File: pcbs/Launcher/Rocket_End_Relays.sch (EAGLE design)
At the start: 39 parts, among them IC2 LM2576T-ADJ, K4 LD105, K5 LD105, K6 LD105, K7 LD105, T1 BC547, T2 BC547, T3 BC547, T4 BC547, T5 BC547, U1 ARDUINO-MEGAPRO-5V, X1 22-23-2041, X2 22-23-2041, X3 22-23-2021, X4 22-23-2021, X5 22-23-2021, X7 22-23-2021

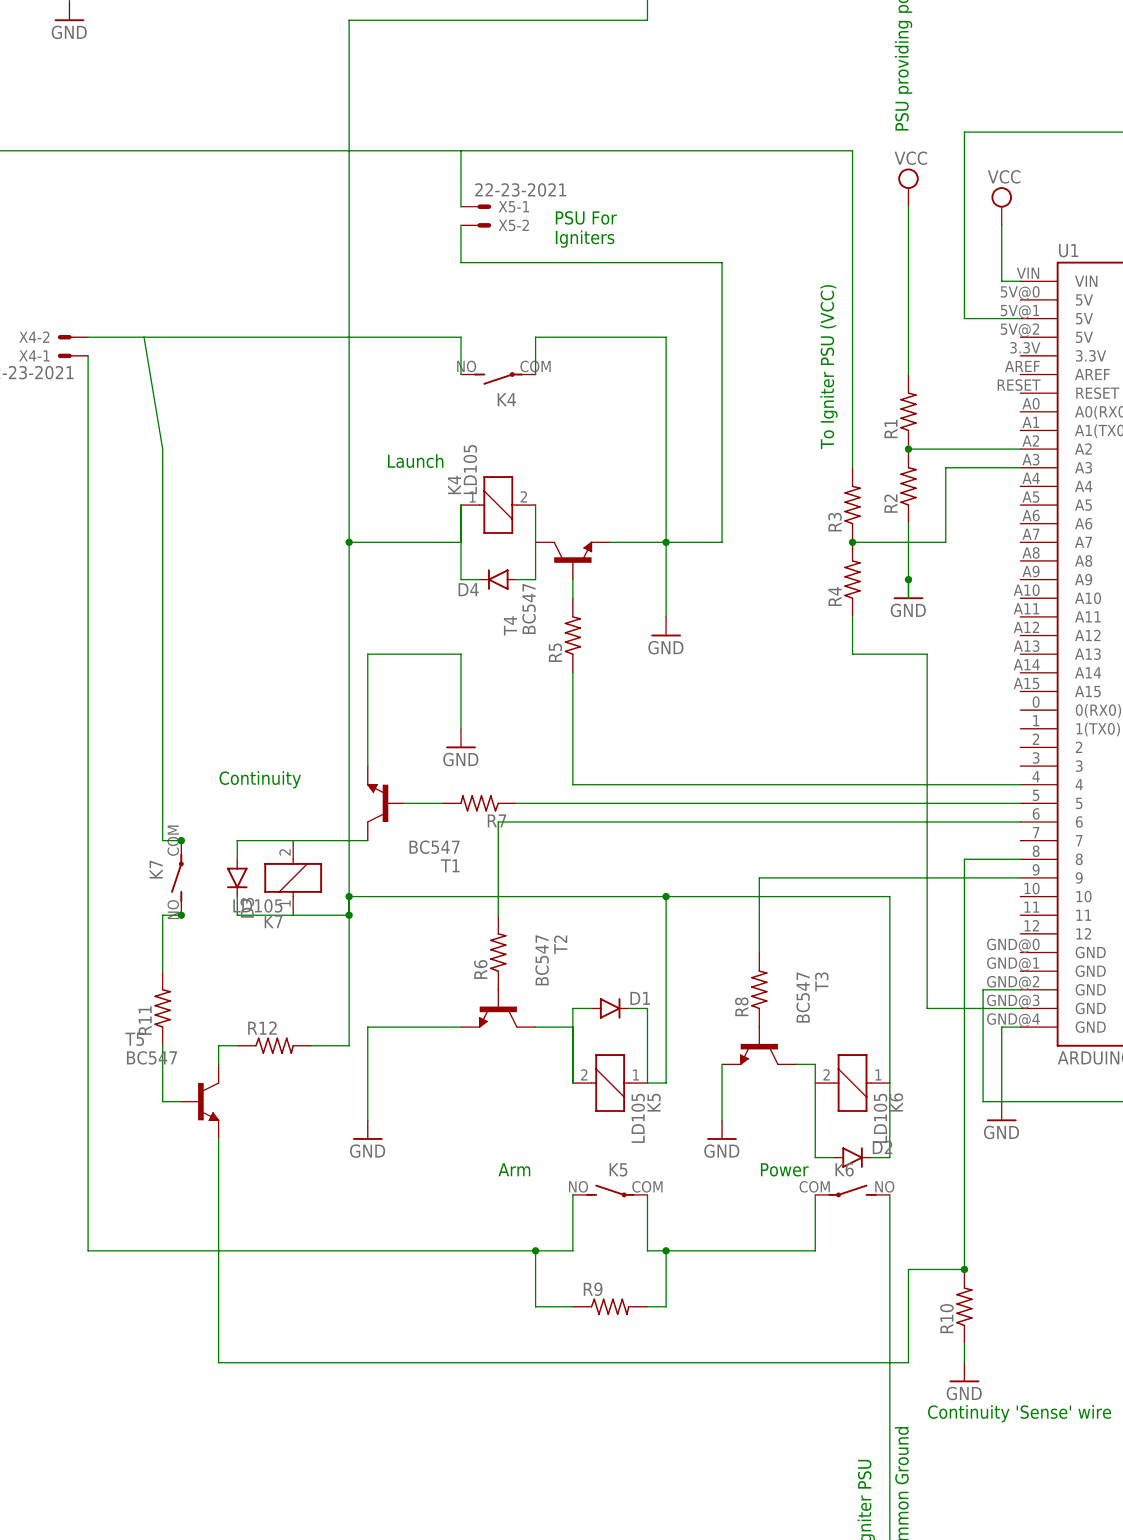
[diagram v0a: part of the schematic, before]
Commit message: * Added Arduino code for launcher code
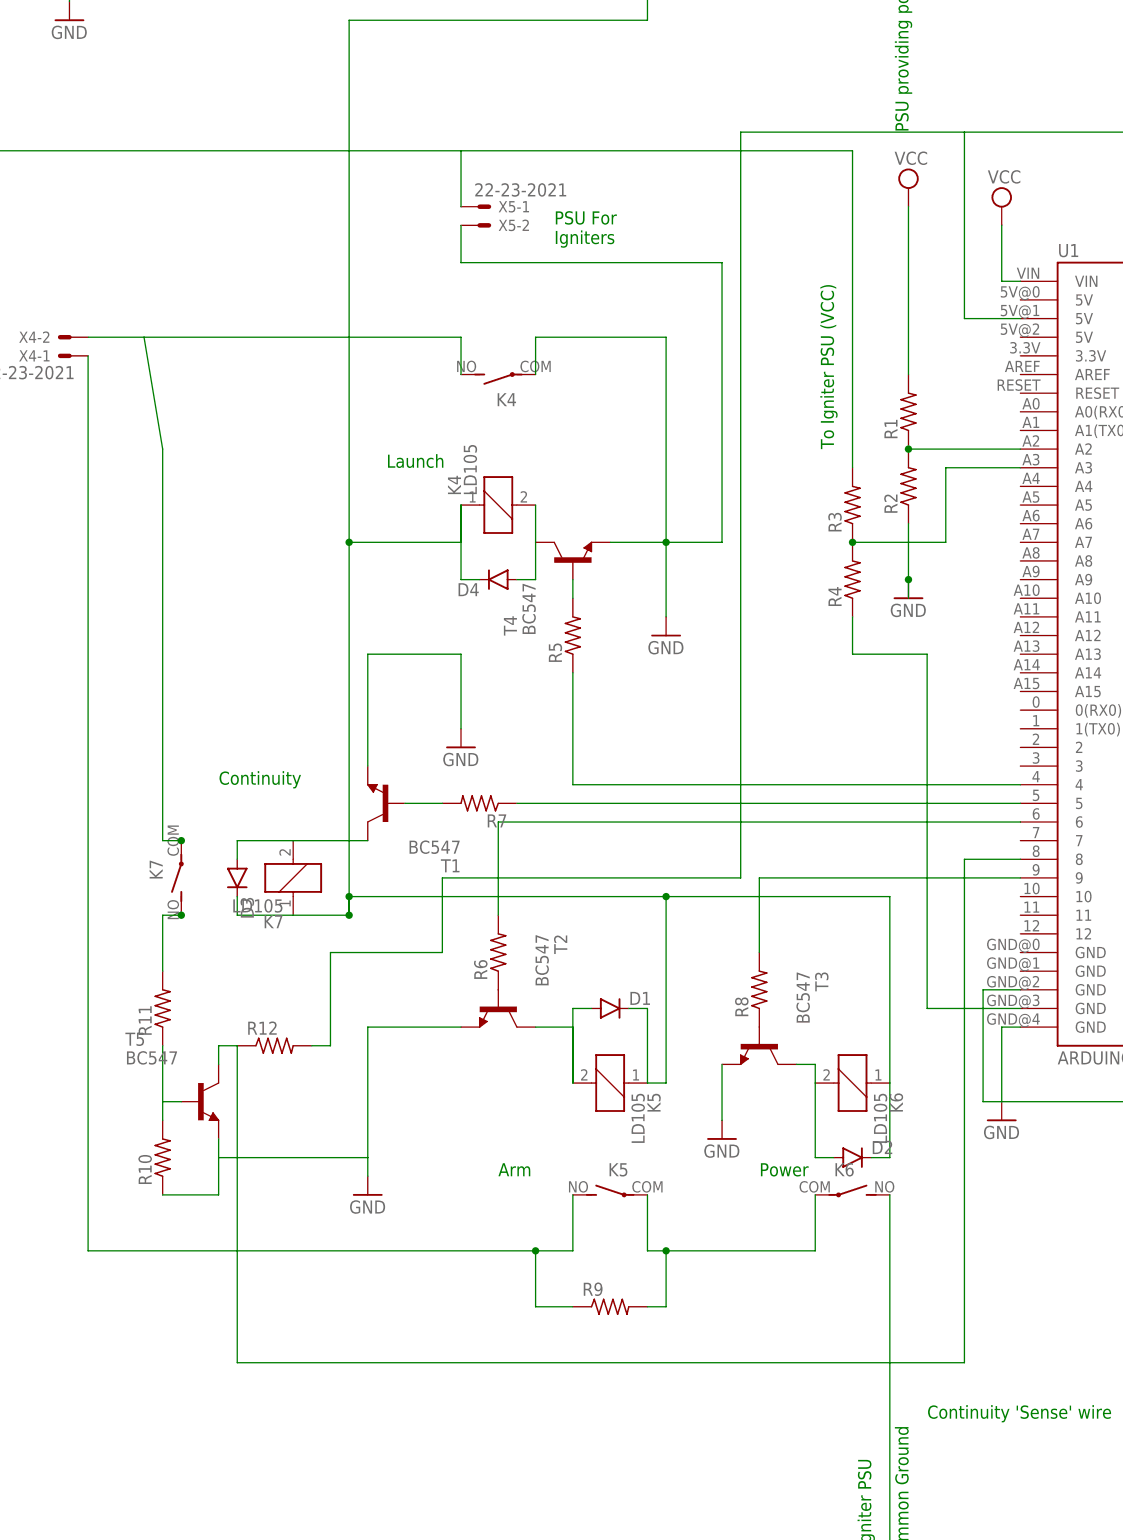
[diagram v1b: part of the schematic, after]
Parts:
- R10: device resistor:R-US_0207/7 -> rcl:R-US_0207/7
- R13, R14: device rcl:R-US_0204/5 -> resistor:R-US_0207/7
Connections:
- removed net N$28: U1.5V@1, X1-3.S, X2-3.S
- net N$23: now also R12.2, U1.5V@1, X1-3.S, X2-3.S; no longer R12.1, T5.C
- net N$26: now also R12.1, T5.C; no longer R10.2, T5.E
- net N$31: now also R10.2
- net N$33: now also T5.E
- net N$5: no longer R12.2
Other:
- moved on the sheet: R10
